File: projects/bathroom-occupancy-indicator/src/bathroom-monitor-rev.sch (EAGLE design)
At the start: 18 parts, among them IC1 7805T, J1 12V, T1 2N2222, U1 ATTINY85-20PU, U2 ATTINY85-20PU

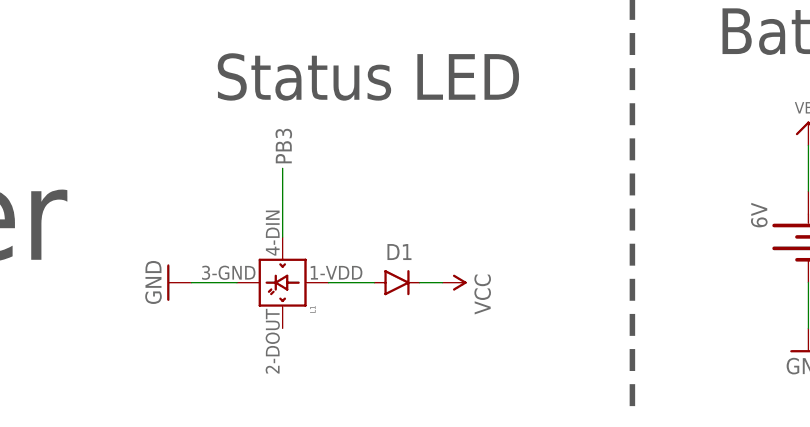
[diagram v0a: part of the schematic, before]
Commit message: pictures cleanup + instructions in progress
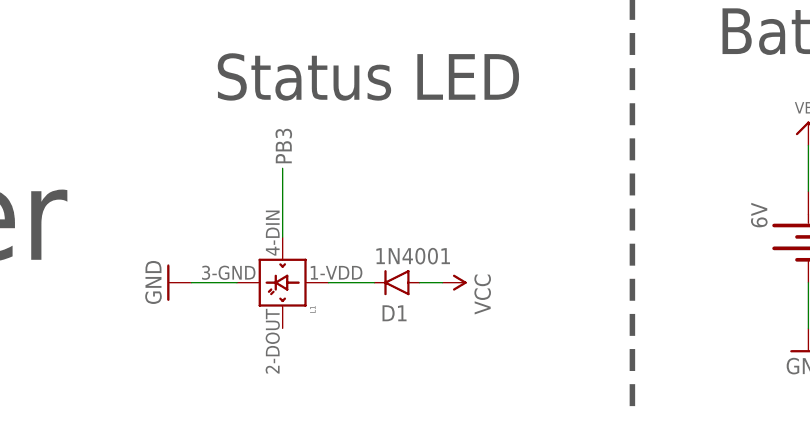
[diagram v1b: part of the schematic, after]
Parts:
- D1: value (none) -> 1N4001
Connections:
- net N$6: now also D1.C; no longer D1.A
- net VCC: now also D1.A; no longer D1.C
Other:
- moved on the sheet: D1
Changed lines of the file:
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@@
 <part name="GND8" library="SparkFun-Aesthetics" deviceset="GND" device=""/>
 <part name="J1" library="con-jack" deviceset="JACK-PLUG" device="1" value="12V"/>
-<part name="D1" library="SparkFun-DiscreteSemi" deviceset="DIODE" device="KIT2"/>
+<part name="D1" library="SparkFun-DiscreteSemi" deviceset="DIODE" device="KIT2" value="1N4001"/>
 <part name="T1" library="adafruit" deviceset="2N2222" device=""/>
 </parts>
@@
 <instance part="GND8" gate="1" x="149.86" y="10.16"/>
 <instance part="J1" gate="G$1" x="22.86" y="109.22"/>
-<instance part="D1" gate="G$1" x="104.14" y="17.78" smashed="yes">
-<attribute name="NAME" x="102.87" y="20.2946" size="1.778" layer="95"/>
-<attribute name="VALUE" x="106.68" y="15.4686" size="1.778" layer="96"/>
+<instance part="D1" gate="G$1" x="104.14" y="17.78" smashed="yes" rot="R180">
+<attribute name="NAME" x="105.41" y="15.2654" size="1.778" layer="95" rot="R180"/>
+<attribute name="VALUE" x="110.236" y="21.6154" size="1.778" layer="96" rot="R180"/>
 </instance>
 <instance part="T1" gate="G$1" x="198.374" y="100.584" rot="R270"/>
@@
 </segment>
 <segment>
+<pinref part="D1" gate="G$1" pin="A"/>
 <pinref part="SUPPLY3" gate="G$1" pin="VCC"/>
-<pinref part="D1" gate="G$1" pin="C"/>
-<wire x1="109.22" y1="17.78" x2="106.68" y2="17.78" width="0.1524" layer="91"/>
+<wire x1="106.68" y1="17.78" x2="109.22" y2="17.78" width="0.1524" layer="91"/>
 </segment>
 </net>
@@
 </segment>
 </net>
-<net name="N$6" class="0">
-<segment>
-<pinref part="D1" gate="G$1" pin="A"/>
-<pinref part="L1" gate="G$1" pin="VDD"/>
-<wire x1="101.6" y1="17.78" x2="96.52" y2="17.78" width="0.1524" layer="91"/>
-</segment>
-</net>
 <net name="N$8" class="0">
 <segment>
@@
 </segment>
 </net>
+<net name="N$6" class="0">
+<segment>
+<pinref part="D1" gate="G$1" pin="C"/>
+<pinref part="L1" gate="G$1" pin="VDD"/>
+<wire x1="101.6" y1="17.78" x2="96.52" y2="17.78" width="0.1524" layer="91"/>
+</segment>
+</net>
